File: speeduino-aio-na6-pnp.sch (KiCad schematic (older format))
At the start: 5 parts, among them J1 Conn_02x03_Odd_Even, J2 Conn_01x06, U1 ATmega2560-16AU, Y1 Crystal_GND2

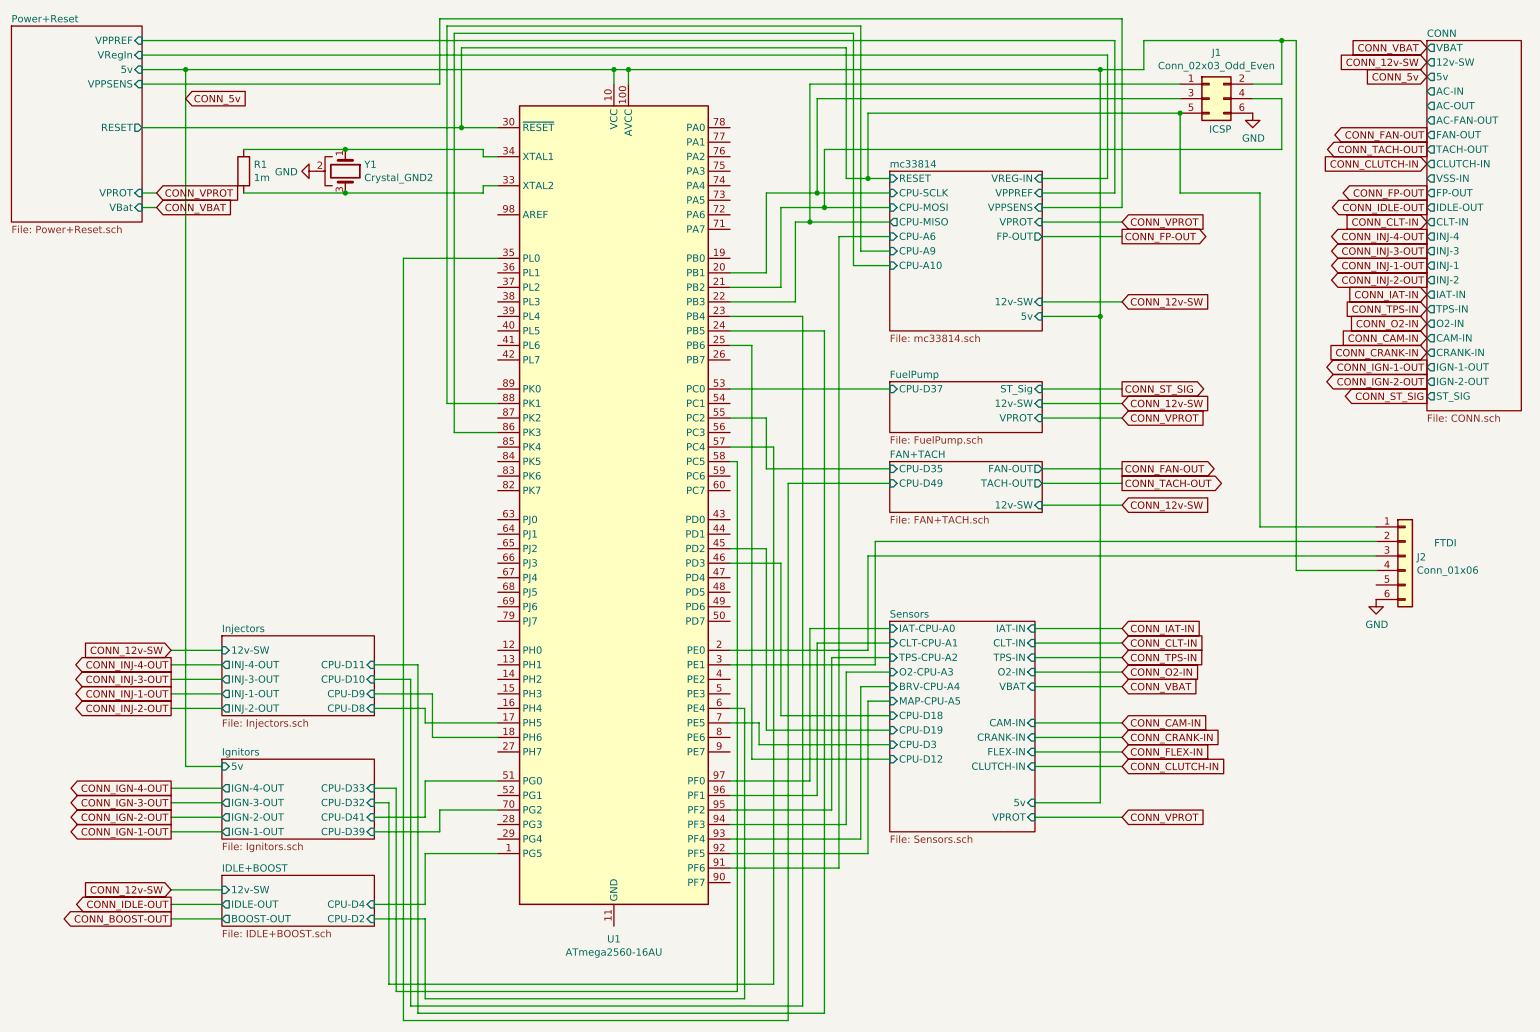
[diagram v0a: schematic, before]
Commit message: restart a third time
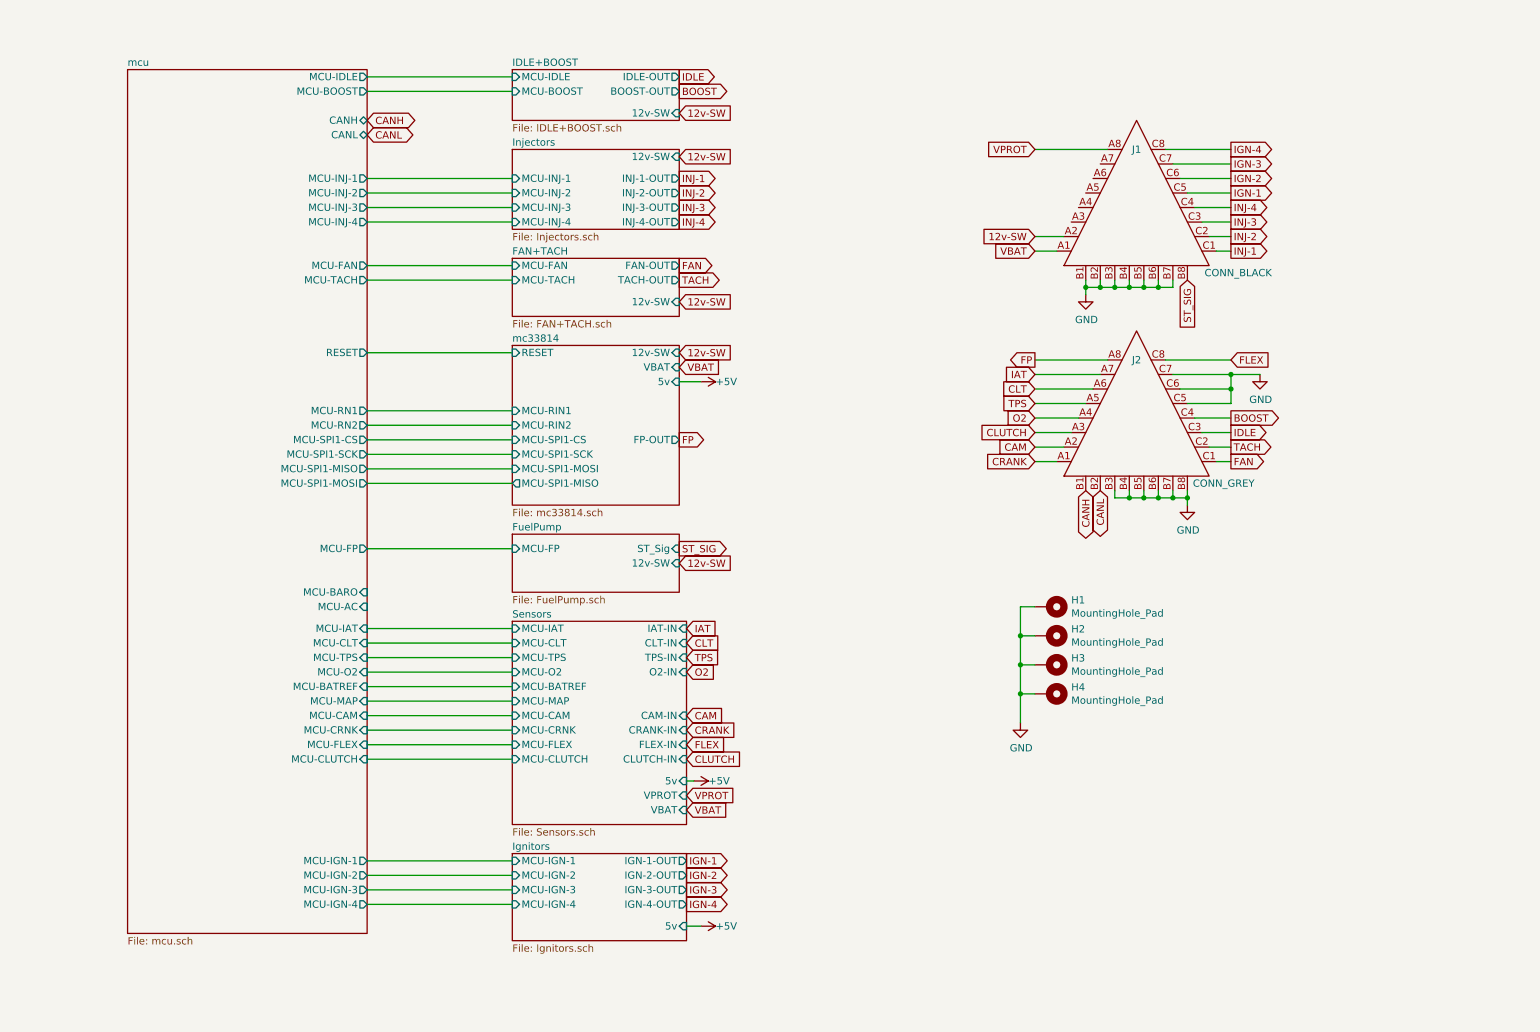
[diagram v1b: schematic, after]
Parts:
- removed J1: Conn_02x03_Odd_Even, Connector_PinHeader_2.54mm:PinHeader_2x03_P2.54mm_Vertical_SMD, symbol Connector_Generic:Conn_02x03_Odd_Even
- removed J2: Conn_01x06, Connector_PinHeader_2.54mm:PinHeader_1x06_P2.54mm_Vertical_SMD_Pin1Left, symbol Connector_Generic:Conn_01x06
- removed R1: 1m, Resistor_SMD:R_0603_1608Metric_Pad1.05x0.95mm_HandSolder, symbol Device:R
- removed U1: ATmega2560-16AU, Package_QFP:TQFP-100_14x14mm_P0.5mm, symbol MCU_Microchip_ATmega:ATmega2560-16AU
- removed Y1: Crystal_GND2, Crystal:Crystal_SMD_3225-4Pin_3.2x2.5mm_HandSoldering, symbol Device:Crystal_GND2
- added H1, H2, H3, H4: MountingHole_Pad, MountingHole:MountingHole_4.3mm_M4_Pad_Via, symbol Mechanical:MountingHole_Pad
- added J1: CONN_BLACK, speeduino_connector_automotive:Delphi_Sicma_24_Black, symbol speeduino_connector_automotive:Delphi_Sicma_24
- added J2: CONN_GREY, speeduino_connector_automotive:Delphi_Sicma_24_Grey, symbol speeduino_connector_automotive:Delphi_Sicma_24
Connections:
- net GND: now also H1.1, H2.1, H3.1, H4.1, J1.B1, J1.B2, J1.B3, J1.B4, J1.B5, J1.B6, J1.B7, J2.B3, J2.B4, J2.B5, J2.B6, J2.B7, J2.B8, J2.C5, J2.C6, J2.C7
- new net 12v-SW: J1.A2
- new net BOOST: J2.C4
- new net CAM: J2.A2
- new net CANH: J2.B1
- new net CANL: J2.B2
- new net CLT: J2.A6
- new net CLUTCH: J2.A3
- new net CRANK: J2.A1
- new net FAN: J2.C1
- new net FLEX: J2.C8
- new net FP: J2.A8
- new net IAT: J2.A7
- new net IDLE: J2.C3
- new net IGN-1: J1.C5
- new net IGN-2: J1.C6
- new net IGN-3: J1.C7
- new net IGN-4: J1.C8
- new net INJ-1: J1.C1
- new net INJ-2: J1.C2
- new net INJ-3: J1.C3
- new net INJ-4: J1.C4
- new net O2: J2.A4
- new net ST_SIG: J1.B8
- new net TACH: J2.C2
- new net TPS: J2.A5
- new net VBAT: J1.A1
- new net VPROT: J1.A8
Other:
- note removed: "FTDI"
- note removed: "ICSP"
